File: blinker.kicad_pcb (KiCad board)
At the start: 2 copper layers, 27.8 x 32 mm, 32 parts, among them Q1 NTR4003NT3G, Q2 NTR4003NT3G, Q3 NTR4003NT3G, Q4 NTR4003NT3G, t2 TEST_1P

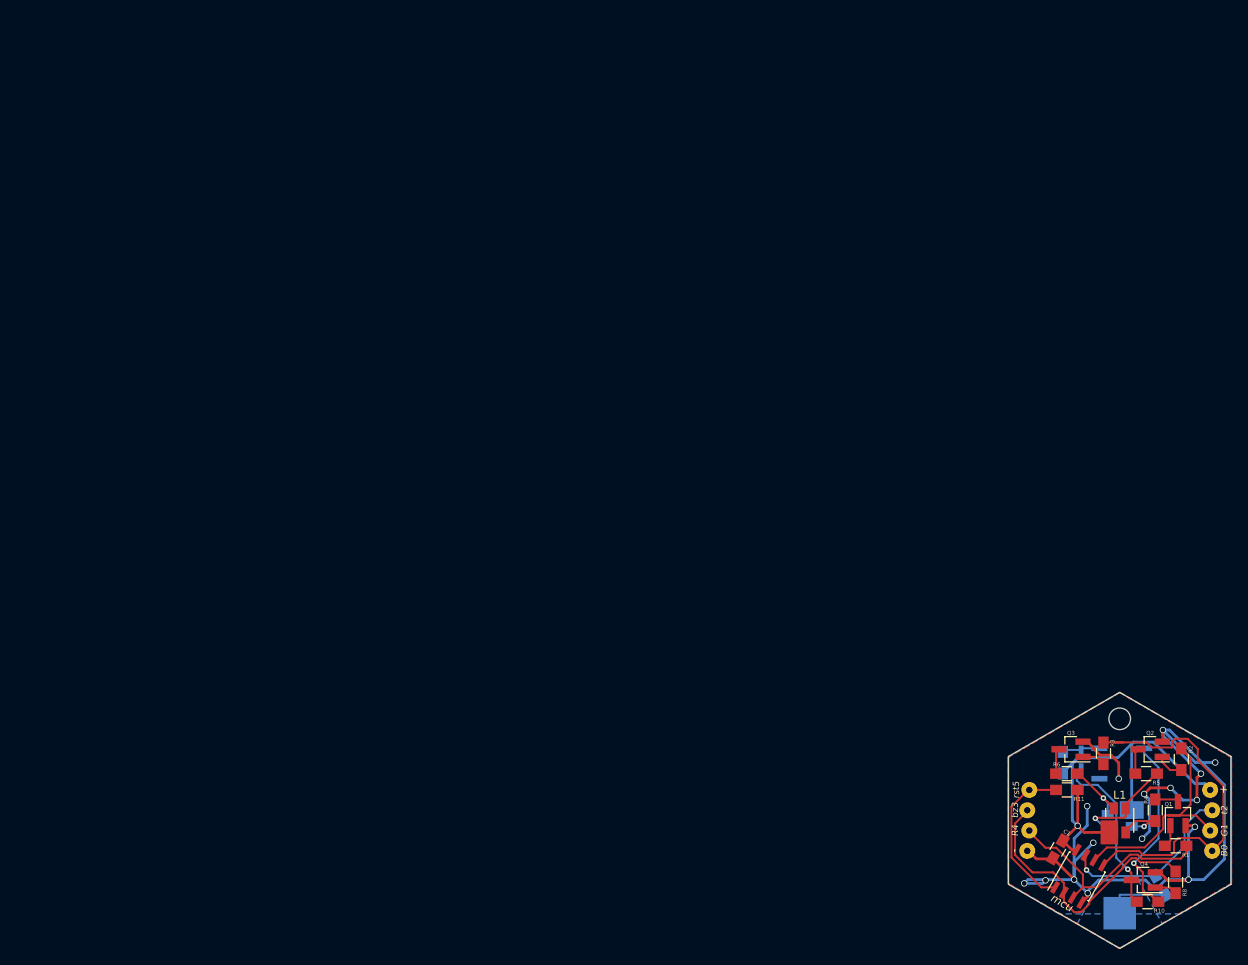
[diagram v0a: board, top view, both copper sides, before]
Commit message: 2 version, already built, ready to be tested
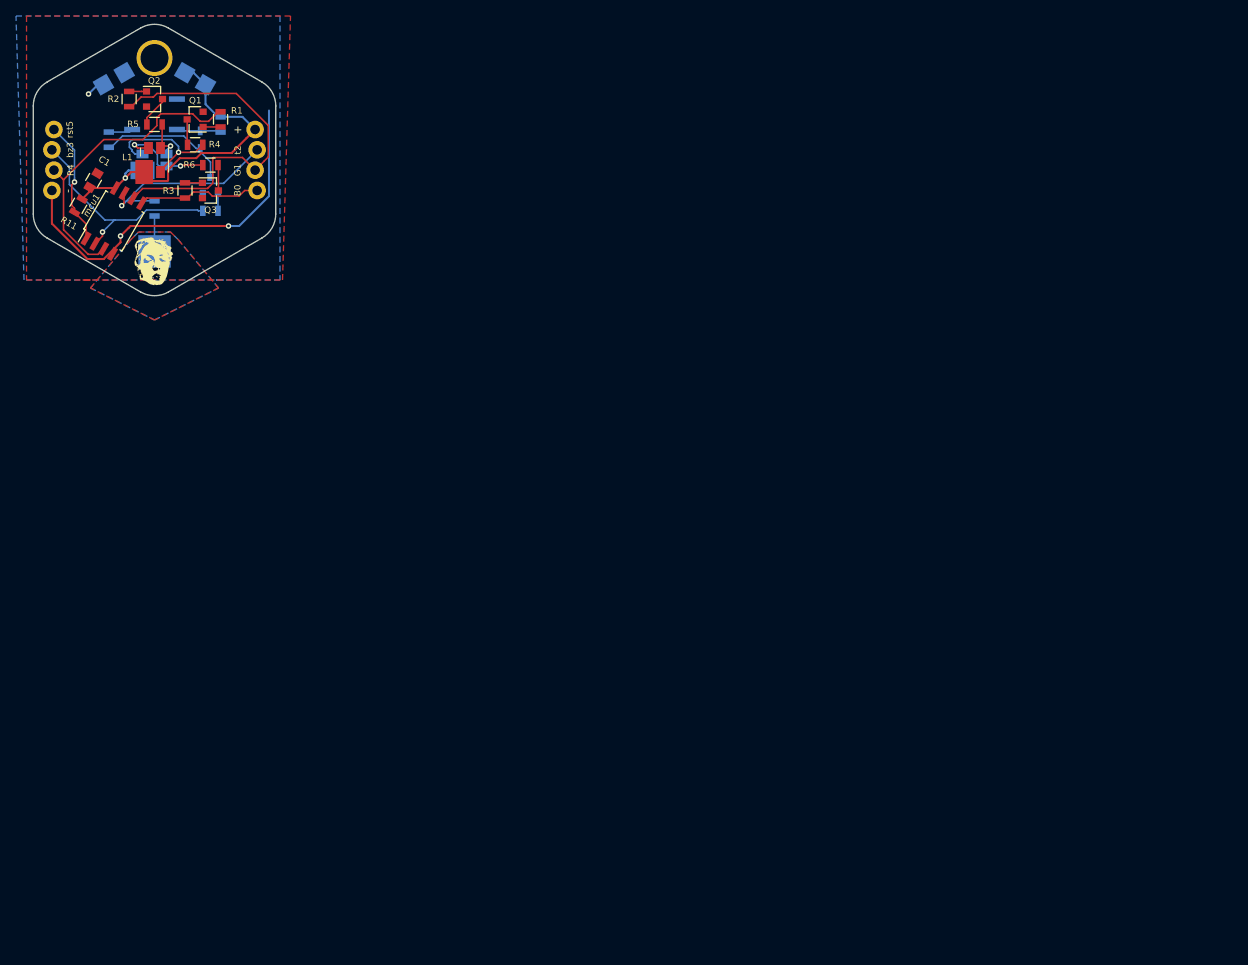
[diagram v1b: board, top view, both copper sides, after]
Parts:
- removed the + at (132.0, 78.7)
- removed the - at (109.1, 86.4)
- removed the R4 at (109.3, 83.8)
- removed the R4 at (125.1, 81.3)
- removed the REF** at (120.7, 69.8)
- removed click: TOUCH_PAD_COPPER, SMD_Packages:1Pin
- removed mcu: ATTINY85V-10SU, Housings_SOIC:SOIC-8_3.9x4.9mm_Pitch1.27mm
- added +: TEST_1P, Wire_Pads:SolderWirePad_single_1-2mmDrill, F.Cu at (12.6, -3.81)
- added +: TEST_1P, wrirepad:singlesolderpad, B.Cu at (5.08, -10.2)
- added -: TEST_1P, Wire_Pads:SolderWirePad_single_1-2mmDrill, F.Cu at (-12.8, 3.81)
- added -: TEST_1P, wrirepad:singlesolderpad, B.Cu at (-5.08, -10.2)
- added G***: LOGO, blinker_attiny85:italia, B.Cu at (-11.0, 7.00)
- added J9: TOUCH_PAD_COPPER, SMD_Packages:1Pin, B.Cu at (0.00, 11.4)
- added R4: 33R, Resistors_SMD:R_0805, F.Cu at (5.08, -1.91)
- added R4: TEST_1P, Wire_Pads:SolderWirePad_single_1-2mmDrill, F.Cu at (-12.6, 1.27)
- added REF**: SolderWirePad_single_2mmDrill, Wire_Pads:SolderWirePad_single_2mmDrill, F.Cu at (0.00, -12.8)
- added mcu1: ATTINY85V-10SU, Housings_SOIC:SOIJ-8_5.3x5.3mm_Pitch1.27mm, F.Cu at (-5.08, 7.62)
- B0, G1, bz3, rst5, t2: footprint Wire_Pads:SolderWirePad_single_0-8mmDrill -> Wire_Pads:SolderWirePad_single_1-2mmDrill
- C1: footprint Capacitors_SMD:C_0805_HandSoldering -> Capacitors_SMD:C_0805
- G***: moved to F.Cu
- Q1, Q2, Q3: footprint TO_SOT_Packages_SMD:SOT-23_Handsoldering -> TO_SOT_Packages_SMD:SOT-23
- Q4: footprint TO_SOT_Packages_SMD:SOT-23_Handsoldering -> TO_SOT_Packages_SMD:SOT-23; moved to B.Cu
- R1, R11, R2, R3, R7: footprint Resistors_SMD:R_0805_HandSoldering -> Resistors_SMD:R_0805
- R10: value 27R -> 33R; footprint Resistors_SMD:R_0805_HandSoldering -> Resistors_SMD:R_0805; moved to B.Cu
- R5, R6: value 34R -> 33R; footprint Resistors_SMD:R_0805_HandSoldering -> Resistors_SMD:R_0805
- R8: footprint Resistors_SMD:R_0805_HandSoldering -> Resistors_SMD:R_0805; moved to B.Cu
- R9: value 10K -> 20K; footprint Resistors_SMD:R_0805_HandSoldering -> Resistors_SMD:R_0805
- moved R10 161.0 mm to (-5.71, -2.54), turned to 90 degrees
- moved R2 155.3 mm to (-3.17, -7.62), turned to 270 degrees
- moved R9 151.6 mm to (0.00, 6.05), turned to 270 degrees
- moved Q1 150.4 mm to (5.08, -5.08), turned to 180 degrees
- moved R1 150.0 mm to (8.26, -5.08), turned to 90 degrees
- moved Q2 148.6 mm to (0.00, -7.62), turned to 0 degrees
- moved R5 148.2 mm to (0.00, -4.45)
- moved bz3 147.2 mm to (-12.8, -1.27), turned to 270 degrees
- moved rst5 147.2 mm to (-12.6, -3.81), turned to 270 degrees
- moved R8 147.0 mm to (6.99, 6.35), turned to 180 degrees
- moved C1 146.7 mm to (-7.62, 2.54), turned to 60 degrees
- moved L1 146.2 mm to (0.00, 0.00)
- moved L2 146.2 mm to (0.00, 0.00), turned to 90 degrees
- moved BZ1 145.6 mm to (0.00, -5.71), turned to 180 degrees
- moved Q4 145.4 mm to (6.99, 3.17), turned to 90 degrees
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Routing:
- net GND: track 130.4 -> 49.9 mm, vias 16 -> 3
- net /BLUE: track 46.0 -> 15.5 mm
- net Net-(BZ1-Pad2): track 22.8 -> 3.05 mm, vias 1 -> 0
- net /GREEN: track 29.5 -> 45.9 mm
- net /RED: track 28.5 -> 39.2 mm
- net VCC: track 54.0 -> 43.4 mm
- net /RED_MOS: track 7.63 -> 16.9 mm
- net /GREEN_MOS: track 12.9 -> 5.59 mm
- net /BUZZER: track 34.5 -> 28.3 mm, vias 0 -> 1
- net Net-(D1-Pad2): track 21.7 -> 16.8 mm, vias 1 -> 0
- net /RESET: track 19.8 -> 15.6 mm, vias 0 -> 1
- net /BLUE_MOS: track 8.57 -> 12.4 mm, vias 1 -> 2
- net Net-(J9-Pad1): track 8.05 -> 4.43 mm
- net /TOUCH: track 22.9 -> 25.8 mm
- net Net-(Q2-Pad1): track 3.50 -> 2.17 mm
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- added copper zone on F.Cu, net Net-(J9-Pad1)
- removed copper zone on F.Cu, net (none)
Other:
- board size 27.8 x 32 mm -> 30.3 x 33.9 mm
- net class 0.2mm added: clearance 0.2, trace_width 0.2, via_dia 0.6858, via_drill 0.3302
- net class Default: clearance 0.1524 -> 0.254; trace_width 0.1524 -> 0.254
- net class Minimal added: clearance 0.1524, trace_width 0.1524, via_dia 0.6858, via_drill 0.3302
- net class pwr removed
- rule pad_to_mask_clearance: 0.2 -> 0.05
- rule trace_clearance: 0.1524 -> 0.254
- board text added: "click"
- board text removed: "+"
- board text removed: "-"
- board text removed: "B0"
- board text removed: "G1"
- board text removed: "R4"
- board text removed: "Sul on ilus naeratus"
- board text removed: "bz3"
- board text removed: "rst5"
- board text removed: "t2"
